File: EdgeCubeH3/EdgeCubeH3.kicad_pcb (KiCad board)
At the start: 2 copper layers, 52 x 52 mm, 19 parts, among them U1 H3, U2 K4B4G1646Q

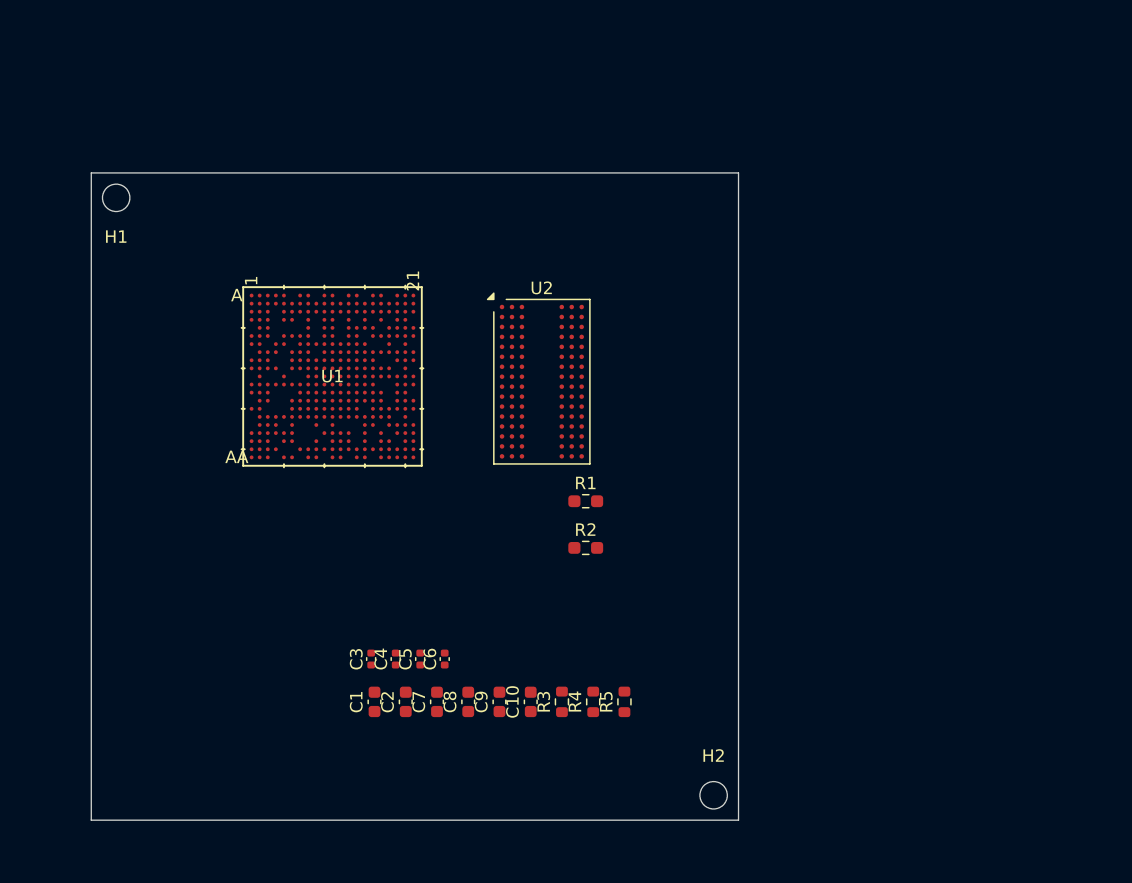
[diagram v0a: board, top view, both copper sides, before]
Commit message: Schematic update, PCB started
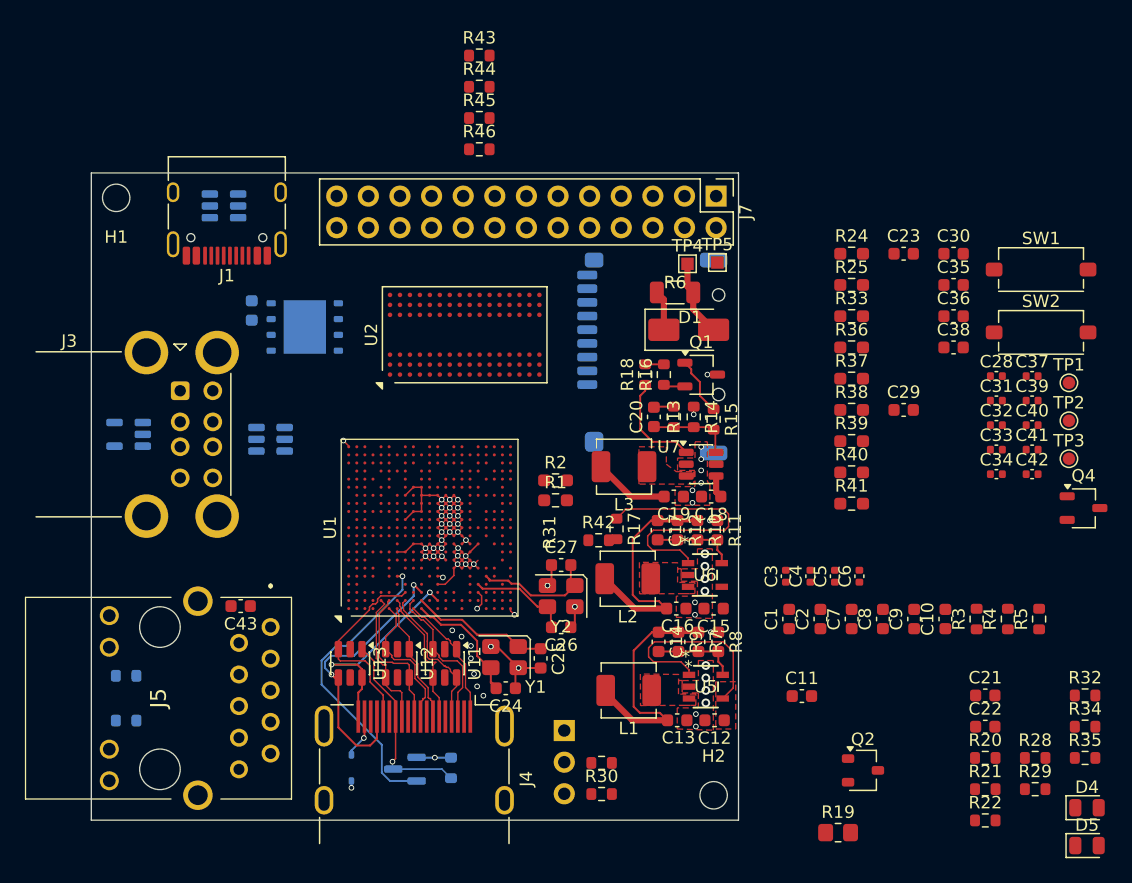
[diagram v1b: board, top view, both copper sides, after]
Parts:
- added C11: 1u, Capacitor_SMD:C_0603_1608Metric, F.Cu at (184.1, 120.0)
- added C12: 10u, Capacitor_SMD:C_0603_1608Metric, F.Cu at (177.1, 122.0)
- added C13: 10u, Capacitor_SMD:C_0603_1608Metric, F.Cu at (174.1, 122.0)
- added C14: 22p, Capacitor_SMD:C_0603_1608Metric, F.Cu at (172.6, 115.7)
- added C15: 10u, Capacitor_SMD:C_0603_1608Metric, F.Cu at (177.0, 113.0)
- added C16: 10u, Capacitor_SMD:C_0603_1608Metric, F.Cu at (174.0, 113.0)
- added C17: 22p, Capacitor_SMD:C_0603_1608Metric, F.Cu at (172.5, 106.7)
- added C18: 10u, Capacitor_SMD:C_0603_1608Metric, F.Cu at (176.8, 104.0)
- added C19: 10u, Capacitor_SMD:C_0603_1608Metric, F.Cu at (173.8, 104.0)
- added C20: 15p, Capacitor_SMD:C_0603_1608Metric, F.Cu at (172.2, 97.6)
- added C21: 2u2, Capacitor_SMD:C_0603_1608Metric, F.Cu at (198.8, 120.0)
- added C22: 2u2, Capacitor_SMD:C_0603_1608Metric, F.Cu at (198.8, 122.5)
- added C23: 4u7, Capacitor_SMD:C_0603_1608Metric, F.Cu at (192.3, 84.5)
- added C24: 15p, Capacitor_SMD:C_0603_1608Metric, F.Cu at (160.3, 119.4)
- added C25: 15p, Capacitor_SMD:C_0603_1608Metric, F.Cu at (163.1, 117.0)
- added C26: 15p, Capacitor_SMD:C_0603_1608Metric, F.Cu at (164.8, 114.5)
- added C27: 15p, Capacitor_SMD:C_0603_1608Metric, F.Cu at (164.8, 109.5)
- added C28: 100n, Capacitor_SMD:C_0402_1005Metric, F.Cu at (199.7, 94.3)
- added C29: 4u7, Capacitor_SMD:C_0603_1608Metric, F.Cu at (192.3, 97.0)
- added C30: 100n, Capacitor_SMD:C_0603_1608Metric, F.Cu at (196.3, 84.5)
- added C31: 100n, Capacitor_SMD:C_0402_1005Metric, F.Cu at (199.7, 96.3)
- added C32: 100n, Capacitor_SMD:C_0402_1005Metric, F.Cu at (199.7, 98.3)
- added C33: 100n, Capacitor_SMD:C_0402_1005Metric, F.Cu at (199.7, 100.2)
- added C34: 100n, Capacitor_SMD:C_0402_1005Metric, F.Cu at (199.7, 102.2)
- added C35: 10u, Capacitor_SMD:C_0603_1608Metric, F.Cu at (196.3, 87.0)
- added C36: 10u, Capacitor_SMD:C_0603_1608Metric, F.Cu at (196.3, 89.5)
- added C37: 100n, Capacitor_SMD:C_0402_1005Metric, F.Cu at (202.6, 94.3)
- added C38: 10u, Capacitor_SMD:C_0603_1608Metric, F.Cu at (196.3, 92.0)
- added C39: 100n, Capacitor_SMD:C_0402_1005Metric, F.Cu at (202.6, 96.3)
- added C40: 100n, Capacitor_SMD:C_0402_1005Metric, F.Cu at (202.6, 98.3)
- added C41: 100n, Capacitor_SMD:C_0402_1005Metric, F.Cu at (202.6, 100.2)
- added C42: 100n, Capacitor_SMD:C_0402_1005Metric, F.Cu at (202.6, 102.2)
- added C43: 1u, Capacitor_SMD:C_0603_1608Metric, F.Cu at (139.0, 112.8)
- added C44: 1u, Capacitor_SMD:C_0603_1608Metric, B.Cu at (139.9, 89.0)
- added D1: SS12, Diode_SMD:D_SMA, F.Cu at (175.0, 90.6)
- added D2: 1N5819WS, Diode_SMD:D_SOD-323, B.Cu at (147.9, 125.8)
- added D4: LED, LED_SMD:LED_0805_2012Metric, F.Cu at (207.0, 129.0)
- added D5: LED, LED_SMD:LED_0805_2012Metric, F.Cu at (207.0, 132.0)
- added J1: USB PWR, Connector_USB:USB_C_Receptacle_HRO_TYPE-C-31-M-12, F.Cu at (137.9, 80.6)
- added J3: USB_A_Stacked, Connector_USB:USB_A_CUI_UJ2-ADH-TH_Horizontal_Stacked, F.Cu at (134.1, 95.5)
- added J4: GPDI_A, Connector_Video:HDMI_A_Molex_208658-1001_Horizontal, F.Cu at (152.9, 125.0)
- added J5: 93626-3006, rj45:936263006, F.Cu at (141.4, 114.5)
- added J6: DBG UART, Connector_PinHeader_2.54mm:PinHeader_1x03_P2.54mm_Vertical, B.Cu at (165.0, 122.8)
- added J7: GPIO, Connector_PinHeader_2.54mm:PinHeader_2x13_P2.54mm_Vertical, F.Cu at (177.2, 79.9)
- added J8: Micro_SD_Card_Det1, icepi:microSD_TF-01A, B.Cu at (172.2, 93.1)
- added L1: 2u2, Inductor_SMD:L_APV_APH0420, F.Cu at (170.2, 119.6)
- added L2: 2u2, Inductor_SMD:L_APV_APH0420, F.Cu at (170.1, 110.6)
- added L3: 2u2, Inductor_SMD:L_APV_APH0420, F.Cu at (169.8, 101.6)
- added Q1: NPN, Package_TO_SOT_SMD:TSOT-23, F.Cu at (176.0, 94.2)
- added Q2: PMOS, Package_TO_SOT_SMD:SOT-23W, F.Cu at (189.0, 126.0)
- added Q3: AO3404, Package_TO_SOT_SMD:SOT-23, B.Cu at (152.2, 125.9)
- added Q4: NPN, Package_TO_SOT_SMD:TSOT-23, F.Cu at (206.7, 104.9)
- added R10: 200K, Capacitor_SMD:C_0603_1608Metric, F.Cu at (175.7, 106.7)
- added R11: 100K, Capacitor_SMD:C_0603_1608Metric, F.Cu at (177.3, 106.7)
- added R12: 300K, Capacitor_SMD:C_0603_1608Metric, F.Cu at (174.1, 106.7)
- added R13: 10K, Resistor_SMD:R_0603_1608Metric, F.Cu at (173.8, 97.6)
- added R14: 12K, Resistor_SMD:R_0603_1608Metric, F.Cu at (175.4, 97.6)
- added R15: 33K, Resistor_SMD:R_0603_1608Metric, F.Cu at (177.0, 97.8)
- added R16: 33K, Resistor_SMD:R_0603_1608Metric, F.Cu at (173.0, 94.2)
- added R17: 10K, Resistor_SMD:R_0603_1608Metric, F.Cu at (169.2, 106.6)
- added R18: 10K, Resistor_SMD:R_0603_1608Metric, F.Cu at (171.5, 94.2)
- added R19: 100K, Resistor_SMD:R_0805_2012Metric_Pad1.20x1.40mm_HandSolder, F.Cu at (187.0, 131.0)
- added R20: 5K6, Resistor_SMD:R_0603_1608Metric, F.Cu at (198.8, 125.0)
- added R21: 2K, Resistor_SMD:R_0603_1608Metric, F.Cu at (198.8, 127.5)
- added R22: 2K, Resistor_SMD:R_0603_1608Metric, F.Cu at (198.8, 130.0)
- added R23: 30K, Resistor_SMD:R_0603_1608Metric, B.Cu at (155.9, 125.8)
- added R24: 5K6, Resistor_SMD:R_0603_1608Metric_Pad0.98x0.95mm_HandSolder, F.Cu at (188.1, 84.5)
- added R25: 470R, Resistor_SMD:R_0603_1608Metric_Pad0.98x0.95mm_HandSolder, F.Cu at (188.1, 87.0)
- added R26: 470R, Resistor_SMD:R_0603_1608Metric, B.Cu at (129.8, 122.0)
- added R27: 470R, Resistor_SMD:R_0603_1608Metric, B.Cu at (129.8, 118.4)
- added R28: 470R, Resistor_SMD:R_0603_1608Metric, F.Cu at (202.8, 125.0)
- added R29: 470R, Resistor_SMD:R_0603_1608Metric, F.Cu at (202.8, 127.5)
- added R30: 120R, Resistor_SMD:R_0603_1608Metric, F.Cu at (168.0, 127.9)
- added R31: 120R, Resistor_SMD:R_0603_1608Metric, F.Cu at (168.0, 125.4)
- added R32: 10K, Resistor_SMD:R_0603_1608Metric, F.Cu at (206.8, 120.0)
- added R33: 33R, Resistor_SMD:R_0603_1608Metric_Pad0.98x0.95mm_HandSolder, F.Cu at (188.1, 89.5)
- added R34: 47K, Resistor_SMD:R_0603_1608Metric, F.Cu at (206.8, 122.5)
- added R35: 47K, Resistor_SMD:R_0603_1608Metric, F.Cu at (206.8, 125.0)
- added R36: 56K, Resistor_SMD:R_0603_1608Metric_Pad0.98x0.95mm_HandSolder, F.Cu at (188.1, 92.0)
- added R37: 10K, Resistor_SMD:R_0603_1608Metric_Pad0.98x0.95mm_HandSolder, F.Cu at (188.1, 94.5)
- added R38: 10K, Resistor_SMD:R_0603_1608Metric_Pad0.98x0.95mm_HandSolder, F.Cu at (188.1, 97.0)
- added R39: 10K, Resistor_SMD:R_0603_1608Metric_Pad0.98x0.95mm_HandSolder, F.Cu at (188.1, 99.5)
- added R40: 51K, Resistor_SMD:R_0603_1608Metric_Pad0.98x0.95mm_HandSolder, F.Cu at (188.1, 102.1)
- added R41: 51K, Resistor_SMD:R_0603_1608Metric_Pad0.98x0.95mm_HandSolder, F.Cu at (188.1, 104.6)
- added R42: 10M, Resistor_SMD:R_0603_1608Metric, F.Cu at (167.8, 107.5)
- added R43: 3K, Resistor_SMD:R_0603_1608Metric, F.Cu at (158.2, 68.6)
- added R44: 3K, Resistor_SMD:R_0603_1608Metric, F.Cu at (158.2, 71.1)
- added R45: 3K, Resistor_SMD:R_0603_1608Metric, F.Cu at (158.2, 73.6)
- added R46: 3K, Resistor_SMD:R_0603_1608Metric, F.Cu at (158.2, 76.1)
- added R6: 10R, Resistor_SMD:R_1206_3216Metric, F.Cu at (173.9, 87.6)
- added R7: 680K, Capacitor_SMD:C_0603_1608Metric, F.Cu at (175.8, 115.7)
- added R8: 75K, Capacitor_SMD:C_0603_1608Metric, F.Cu at (177.4, 115.7)
- added R9: 680K, Capacitor_SMD:C_0603_1608Metric, F.Cu at (174.2, 115.7)
- added SW1: RST, Button_Switch_SMD:Button_6x3mm, F.Cu at (203.3, 85.8)
- added SW2: PWR, Button_Switch_SMD:Button_6x3mm, F.Cu at (203.3, 90.8)
- added TP1: UBOOT, TestPoint:TestPoint_Pad_D1.0mm, F.Cu at (205.5, 94.9)
- added TP2: PWR_KEY, TestPoint:TestPoint_Pad_D1.0mm, F.Cu at (205.5, 97.9)
- added TP3: TV, TestPoint:TestPoint_Pad_D1.0mm, F.Cu at (205.5, 101.0)
- added TP4: supercap, TestPoint:TestPoint_Pad_1.0x1.0mm, F.Cu at (174.9, 85.3)
- added TP5: gnd, TestPoint:TestPoint_Pad_1.0x1.0mm, F.Cu at (177.3, 85.2)
- added U10: USBLC6-4SC6, Package_TO_SOT_SMD:SOT-23-6, B.Cu at (141.4, 99.4)
- added U11: USBLC6-4SC6, Package_TO_SOT_SMD:SOT-23-6, F.Cu at (155.4, 117.4)
- added U12: USBLC6-4SC6, Package_TO_SOT_SMD:SOT-23-6, F.Cu at (151.6, 117.4)
- added U13: USBLC6-4SC6, Package_TO_SOT_SMD:SOT-23-6, F.Cu at (147.8, 117.4)
- added U3: USBLC6-2SC6, Package_TO_SOT_SMD:SOT-23-6, B.Cu at (137.7, 80.7)
- added U4: SY6280AAC, Package_TO_SOT_SMD:SOT-23-5, B.Cu at (130.0, 99.0)
- added U5: SY8089AAAC, SY8089:SY8089AAAC_SGY, F.Cu at (176.4, 119.3)
- added U6: SY8089AAAC, SY8089:SY8089AAAC_SGY, F.Cu at (176.3, 110.3)
- added U7: SY8032, Package_TO_SOT_SMD:SOT-23-6, F.Cu at (176.0, 101.4)
- added U8: W25Q128JVP, Package_SON:WSON-8-1EP_6x5mm_P1.27mm_EP3.4x4.3mm, B.Cu at (144.2, 90.4)
- added Y1: 24M, Crystal:Crystal_SMD_3225-4Pin_3.2x2.5mm, F.Cu at (160.2, 116.9)
- added Y2: 32K, Crystal:Crystal_SMD_3225-4Pin_3.2x2.5mm, F.Cu at (164.8, 112.0)
- U1: footprint Lib:BGA347_H3_AWT-M -> cm0:FBGA-347_14x14mm_Layout21x21_P0.65mm
- moved C2 34.0 mm to (185.6, 113.8)
- moved C9 34.0 mm to (193.1, 113.8)
- moved C1 34.0 mm to (183.1, 113.8)
- moved C10 34.0 mm to (195.6, 113.8)
- moved C3 34.0 mm to (182.8, 110.4)
- moved C4 34.0 mm to (184.8, 110.4)
- moved C5 34.0 mm to (186.7, 110.4)
- moved C6 34.0 mm to (188.7, 110.4)
- moved C7 34.0 mm to (188.1, 113.8)
- moved C8 34.0 mm to (190.6, 113.8)
- moved R3 34.0 mm to (198.1, 113.8)
- moved R4 34.0 mm to (200.6, 113.8)
- moved R5 34.0 mm to (203.2, 113.8)
- moved U1 14.4 mm to (154.2, 106.5), turned to 90 degrees
- moved U2 7.26 mm to (157.0, 91.0), turned to 90 degrees
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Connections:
- net VDD_DRAM renamed +1V35
- U1 pad A19: unconnected-(U1F-PF1-PadA19) -> /SoC/SDC0_D0
- U1 pad A2: unconnected-(U1D-EPHY_LINK_LED-PadA2) -> /SoC/EPHY_LINK_LED
- U1 pad A21: Net-(U1B-GND-PadA21) -> GND
- U1 pad A3: unconnected-(U1D-EPHY_TXN-PadA3) -> /SoC/EPHY_TX-
- U1 pad A4: unconnected-(U1D-EPHY_RXN-PadA4) -> /SoC/EPHY_RX-
- U1 pad A5: unconnected-(U1E-USB_D0+-PadA5) -> USB_D0+
- U1 pad A7: unconnected-(U1E-USB_D2+-PadA7) -> USB_D2+
- U1 pad A8: unconnected-(U1E-USB_D2--PadA8) -> USB_D2-
- U1 pad AA1: Net-(U1B-GND-PadA21) -> GND
- U1 pad AA6: unconnected-(U1G-NMI-PadAA6) -> Net-(U1G-NMI)
- U1 pad B13: unconnected-(U1F-PA18-PadB13) -> TWI1_SCK
- U1 pad B14: unconnected-(U1F-PA19-PadB14) -> TWI1_SDA
- U1 pad B15: unconnected-(U1C-PC3-PadB15) -> SPI0_CS
- U1 pad B16: unconnected-(U1C-PC2-PadB16) -> SPI0_CLK
- U1 pad B3: unconnected-(U1D-EPHY_TXP-PadB3) -> /SoC/EPHY_TX+
- U1 pad B4: unconnected-(U1D-EPHY_RXP-PadB4) -> /SoC/EPHY_RX+
- U1 pad B5: unconnected-(U1E-USB_D0--PadB5) -> USB_D0-
- U1 pad B6: unconnected-(U1E-USB_D1+-PadB6) -> USB_D1+
- U1 pad B7: unconnected-(U1E-USB_D1--PadB7) -> USB_D1-
- U1 pad C13: unconnected-(U1F-PA12-PadC13) -> TWI0_SDA
- U1 pad C14: unconnected-(U1F-PA17-PadC14) -> STATUS_LED
- U1 pad C15: unconnected-(U1C-PC0-PadC15) -> SPI0_MOSI
- U1 pad C16: unconnected-(U1C-PC1-PadC16) -> SPI0_MISO
- U1 pad C20: unconnected-(U1F-PF5-PadC20) -> /SoC/SDC0_D2
- U1 pad D11: unconnected-(U1F-PA0-PadD11) -> UART2_TX
- U1 pad D15: unconnected-(U1F-PA16-PadD15) -> SPI1_MISO
- U1 pad D19: unconnected-(U1F-PF0-PadD19) -> /SoC/SDC0_D1
- U1 pad D20: unconnected-(U1F-PF2-PadD20) -> Net-(U1F-PF2)
- U1 pad D3: unconnected-(U1C-PG7-PadD3) -> UART1_RX
- U1 pad D5: unconnected-(U1F-PA1-PadD5) -> UART2_RX
- U1 pad D6: unconnected-(U1F-PA2-PadD6) -> UART2_RTS
- U1 pad D8: unconnected-(U1F-PA7-PadD8) -> PA7
- U1 pad E11: unconnected-(U1F-PA10-PadE11) -> PA10
- U1 pad E13: unconnected-(U1F-PA3-PadE13) -> UART2_CTS
- U1 pad E14: unconnected-(U1F-PA6-PadE14) -> PA6
- U1 pad E15: unconnected-(U1F-PA13-PadE15) -> SPI1_CS
- U1 pad E2: unconnected-(U1D-GPDI_CLK--PadE2) -> /SoC/GPDI_CLK-
- U1 pad E21: unconnected-(U1F-PF4-PadE21) -> /SoC/SDC0_D3
- U1 pad F1: unconnected-(U1D-GPDI_D0--PadF1) -> /SoC/GPDI_D0-
- U1 pad F10: unconnected-(U1D-TVOUT-PadF10) -> Net-(U1D-TVOUT)
- U1 pad F11: unconnected-(U1F-PA11-PadF11) -> TWI0_SCK
- U1 pad F14: unconnected-(U1F-PA15-PadF14) -> SPI1_MOSI
- U1 pad F18: unconnected-(U1F-PF3-PadF18) -> /SoC/SDC0_CMD
- U1 pad F2: unconnected-(U1D-GPDI_CLK+-PadF2) -> /SoC/GPDI_CLK+
- U1 pad F5: unconnected-(U1F-PA4-PadF5) -> UART0_TX
- U1 pad F6: unconnected-(U1D-EPHY_RTX-PadF6) -> Net-(U1D-EPHY_RTX)
- U1 pad F7: unconnected-(U1D-EPHY_SPD_LED-PadF7) -> /SoC/EPHY_SPD_LED
- U1 pad F8: unconnected-(U1D-EPHY_VDD-PadF8) -> +1V2
- U1 pad G1: unconnected-(U1D-GPDI_D0+-PadG1) -> /SoC/GPDI_D0+
- U1 pad G10: unconnected-(U1B-VDD-EFUSE-PadG10) -> Net-(U1B-VDD-EFUSE)
- U1 pad G11: unconnected-(U1E-VCC_USB-PadG11) -> VCC_IO
- U1 pad G12: unconnected-(U1F-PA14-PadG12) -> SPI1_CLK
- U1 pad G13: unconnected-(U1B-VCC-IO-PadG13) -> VCC_IO
- U1 pad G14: unconnected-(U1B-VCC-IO-PadG14) -> VCC_IO
- U1 pad G15: unconnected-(U1B-VCC-IO-PadG15) -> VCC_IO
- U1 pad G18: unconnected-(U1F-PF6-PadG18) -> /SoC/SDC0_DET
- U1 pad G2: unconnected-(U1D-GPDI_D1--PadG2) -> /SoC/GPDI_D1-
- U1 pad G4: unconnected-(U1C-PG6-PadG4) -> UART1_TX
- U1 pad G5: unconnected-(U1D-GPDI_CEC-PadG5) -> /SoC/GPDI_CEC
- U1 pad G7: unconnected-(U1D-EPHY_VCC-PadG7) -> +3V3
- U1 pad G8: Net-(U1B-GND-PadA21) -> GND
- U1 pad G9: unconnected-(U1D-V33_TV-PadG9) -> +3V3
- U1 pad H10: unconnected-(U1B-VDD-SYS-PadH10) -> +1V2
- U1 pad H11: unconnected-(U1B-VDD-EFUSEEBP-PadH11) -> +3V3
- U1 pad H12: Net-(U1B-GND-PadA21) -> GND
- U1 pad H13: unconnected-(U1B-VCC-IO-PadH13) -> VCC_IO
- U1 pad H14: unconnected-(U1B-VCC-IO-PadH14) -> VCC_IO
- U1 pad H15: Net-(U1B-GND-PadA21) -> GND
- U1 pad H2: unconnected-(U1D-GPDI_D1+-PadH2) -> /SoC/GPDI_D1+
- U1 pad H3: unconnected-(U1D-GPDI_SCL-PadH3) -> /SoC/GPDI_SCL
- U1 pad H6: unconnected-(U1F-PA5-PadH6) -> UART0_RX
- U1 pad H7: unconnected-(U1C-VCC-PG-PadH7) -> VCC_IO
- U1 pad H8: unconnected-(U1D-GND_TV-PadH8) -> GND
- U1 pad J1: unconnected-(U1D-GPDI_D2+-PadJ1) -> /SoC/GPDI_D2+
- U1 pad J10: unconnected-(U1B-VDD-SYS-PadJ10) -> +1V2
- U1 pad J11: unconnected-(U1B-VDD-SYS-PadJ11) -> +1V2
- U1 pad J12: unconnected-(U1B-VDD-SYS-PadJ12) -> +1V2
- U1 pad J13: Net-(U1B-GND-PadA21) -> GND
- U1 pad J14: unconnected-(U1B-VCC-IO-PadJ14) -> VCC_IO
- U1 pad J15: unconnected-(U1F-VCC_PD-PadJ15) -> VCC_IO
- U1 pad J16: Net-(U1B-GND-PadA21) -> GND
- U1 pad J2: unconnected-(U1D-GPDI_D2--PadJ2) -> /SoC/GPDI_D2-
- U1 pad J6: unconnected-(U1D-GPDI_VCC-PadJ6) -> +3V3
- U1 pad J7: unconnected-(U1B-VDD-CPUS-PadJ7) -> +1V2
- U1 pad J8: unconnected-(U1B-VDD-CPUS-PadJ8) -> +1V2
- U1 pad J9: Net-(U1B-GND-PadA21) -> GND
- U1 pad K1: unconnected-(U1G-X24MOUT-PadK1) -> Net-(U1G-X24MOUT)
- U1 pad K10: unconnected-(U1B-VDD-SYS-PadK10) -> +1V2
- U1 pad K11: unconnected-(U1B-VDD-SYS-PadK11) -> +1V2
- U1 pad K12: unconnected-(U1B-VDD-SYS-PadK12) -> +1V2
- U1 pad K13: Net-(U1B-GND-PadA21) -> GND
- U1 pad K14: Net-(U1B-GND-PadA21) -> GND
- U1 pad K15: Net-(U1B-GND-PadA21) -> GND
- U1 pad K16: Net-(U1B-GND-PadA21) -> GND
- U1 pad K2: unconnected-(U1G-X24MIN-PadK2) -> Net-(U1G-X24MIN)
- U1 pad K3: unconnected-(U1D-GPDI_SDA-PadK3) -> /SoC/GPDI_SDA
- U1 pad K6: unconnected-(U1G-VCC_RTC-PadK6) -> +3V3
- U1 pad K7: Net-(U1B-GND-PadA21) -> GND
- U1 pad K8: Net-(U1B-GND-PadA21) -> GND
- U1 pad K9: Net-(U1B-GND-PadA21) -> GND
- U1 pad L10: unconnected-(U1B-VDD-SYS-PadL10) -> +1V2
- U1 pad L11: unconnected-(U1B-VDD-SYS-PadL11) -> +1V2
- U1 pad L12: unconnected-(U1B-VDD-SYS-PadL12) -> +1V2
- U1 pad L13: unconnected-(U1B-VDD-SYS-PadL13) -> +1V2
- U1 pad L14: unconnected-(U1B-VDD-SYS-PadL14) -> +1V2
- U1 pad L15: Net-(U1B-GND-PadA21) -> GND
- U1 pad L8: Net-(U1B-GND-PadA21) -> GND
- U1 pad L9: Net-(U1B-GND-PadA21) -> GND
- U1 pad M10: Net-(U1B-GND-PadA21) -> GND
- U1 pad M11: Net-(U1B-GND-PadA21) -> GND
- U1 pad M12: Net-(U1B-GND-PadA21) -> GND
- U1 pad M13: Net-(U1B-GND-PadA21) -> GND
- U1 pad M14: Net-(U1B-GND-PadA21) -> GND
- U1 pad M15: Net-(U1B-GND-PadA21) -> GND
- U1 pad M2: unconnected-(U1D-GPDI_HPD-PadM2) -> /SoC/GPDI_HPD
- U1 pad M4: unconnected-(U1G-RTC_VIO-PadM4) -> +1V2
- U1 pad M5: unconnected-(U1D-GPDI_GND-PadM5) -> GND
- U1 pad M6: unconnected-(U1F-PL9-PadM6) -> PWR_DRAM_EN
- U1 pad M7: Net-(U1B-GND-PadA21) -> GND
- U1 pad M8: Net-(U1B-GND-PadA21) -> GND
- U1 pad M9: Net-(U1B-GND-PadA21) -> GND
- U1 pad N10: Net-(U1B-GND-PadA21) -> GND
- U1 pad N11: Net-(U1B-GND-PadA21) -> GND
- U1 pad N12: Net-(U1B-GND-PadA21) -> GND
- U1 pad N13: Net-(U1B-GND-PadA21) -> GND
- U1 pad N14: Net-(U1B-GND-PadA21) -> GND
- U1 pad N15: Net-(U1B-GND-PadA21) -> GND
- U1 pad N2: unconnected-(U1F-PL4-PadN2) -> Net-(U1F-PL4)
- U1 pad N3: unconnected-(U1G-VCC_PLL-PadN3) -> +3V3
- U1 pad N7: Net-(U1B-GND-PadA21) -> GND
- U1 pad N8: unconnected-(U1B-VDD-CPUX-PadN8) -> +1V2
- U1 pad N9: Net-(U1B-GND-PadA21) -> GND
- U1 pad P10: Net-(U1B-GND-PadA21) -> GND
- U1 pad P11: Net-(U1B-GND-PadA21) -> GND
- U1 pad P12: Net-(U1B-GND-PadA21) -> GND
- U1 pad P13: Net-(U1B-GND-PadA21) -> GND
- U1 pad P14: Net-(U1B-GND-PadA21) -> GND
- U1 pad P15: Net-(U1B-GND-PadA21) -> GND
- U1 pad P6: unconnected-(U1B-VDD-CPUX-PadP6) -> +1V2
- U1 pad P7: unconnected-(U1B-VDD-CPUX-PadP7) -> +1V2
- U1 pad P8: unconnected-(U1B-VDD-CPUX-PadP8) -> +1V2
- U1 pad P9: unconnected-(U1B-VDD-CPUX-PadP9) -> +1V2
- U1 pad R1: unconnected-(U1F-PL3-PadR1) -> Net-(U1F-PL3)
- U1 pad R10: Net-(U1B-GND-PadA21) -> GND
- U1 pad R11: Net-(U1B-GND-PadA21) -> GND
- U1 pad R12: Net-(U1B-GND-PadA21) -> GND
- U1 pad R13: Net-(U1B-GND-PadA21) -> GND
- U1 pad R14: Net-(U1B-GND-PadA21) -> GND
- U1 pad R2: unconnected-(U1F-PL5-PadR2) -> VCC_IO_EN
- U1 pad R6: unconnected-(U1B-VDD-CPUX-PadR6) -> +1V2
- U1 pad R7: unconnected-(U1B-VDD-CPUX-PadR7) -> +1V2
- U1 pad R8: unconnected-(U1B-VDD-CPUX-PadR8) -> +1V2
- U1 pad R9: Net-(U1B-GND-PadA21) -> GND
- U1 pad T10: unconnected-(U1G-VDD-CPUFB-PadT10) -> PWR_CPUFB
- U1 pad T11: Net-(U1B-GND-PadA21) -> GND
- U1 pad T2: unconnected-(U1F-PL8-PadT2) -> PWR_STB_EN
- U1 pad T4: unconnected-(U1F-PL6-PadT4) -> CPUX_VSET
- U1 pad T6: unconnected-(U1B-VDD-CPUX-PadT6) -> +1V2
- U1 pad T7: unconnected-(U1B-VDD-CPUX-PadT7) -> +1V2
- U1 pad T8: unconnected-(U1B-VDD-CPUX-PadT8) -> +1V2
- U1 pad T9: unconnected-(U1G-GND-CPUFB-PadT9) -> GND
- U1 pad U3: unconnected-(U1H-AGND-PadU3) -> GND
- U1 pad U4: unconnected-(U1G-X32KOUT-PadU4) -> Net-(U1G-X32KOUT)
- U1 pad U6: unconnected-(U1B-VDD-CPUX-PadU6) -> +1V2
- U1 pad U9: unconnected-(U1B-VDD-CPUX-PadU9) -> +1V2
- U1 pad V2: unconnected-(U1F-PL10-PadV2) -> PWR_LED
- U1 pad V3: unconnected-(U1H-AVCC-PadV3) -> +3V3
- U1 pad V5: unconnected-(U1G-X32KIN-PadV5) -> Net-(U1G-X32KIN)
- U1 pad V6: unconnected-(U1G-RESET-PadV6) -> /SoC/RESET
- U1 pad W6: unconnected-(U1G-UBOOT-PadW6) -> Net-(U1G-UBOOT)
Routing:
- net GND: track 0.00 -> 64.4 mm, vias 0 -> 53
- net /SoC/GPDI_CEC: track 0.00 -> 24.5 mm, vias 0 -> 1
- net /SoC/GPDI_SDA: track 0.00 -> 22.7 mm, vias 0 -> 2
- net PWR_DRAM_EN: track 0.00 -> 22.1 mm
- net VBUS: track 0.00 -> 21.8 mm, vias 0 -> 1
- net +3V3: track 0.00 -> 21.5 mm
- net +1V35: track 0.00 -> 20.1 mm
- net +1V2: track 0.00 -> 19.8 mm, vias 0 -> 6
- net /SoC/GPDI_HPD: track 0.00 -> 17.7 mm, vias 0 -> 2
- net /SoC/GPDI_SCL: track 0.00 -> 16.0 mm
- net /ports/CEC: track 0.00 -> 15.8 mm, vias 0 -> 1
- net /SoC/GPDI_D2-: track 0.00 -> 12.2 mm
- net /SoC/GPDI_D1+: track 0.00 -> 11.9 mm
- net /SoC/GPDI_CLK+: track 0.00 -> 11.9 mm
- net /SoC/GPDI_D0-: track 0.00 -> 11.5 mm
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- added copper zone on F.Cu, net GND
- added copper zone on In1.Cu, net GND
- added copper zone on In4.Cu, net GND
- added copper zone on F.Cu, net Net-(U5-LX)
- added copper zone on F.Cu, net Net-(U6-LX)
- added copper zone on F.Cu, net Net-(U7-LX)
- added copper zone on F.Cu, net VBUS
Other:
- copper layers 2 -> 6

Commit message: PCB design at ~90%
- re-arrangement of components
- connecting dram
- connecting ports
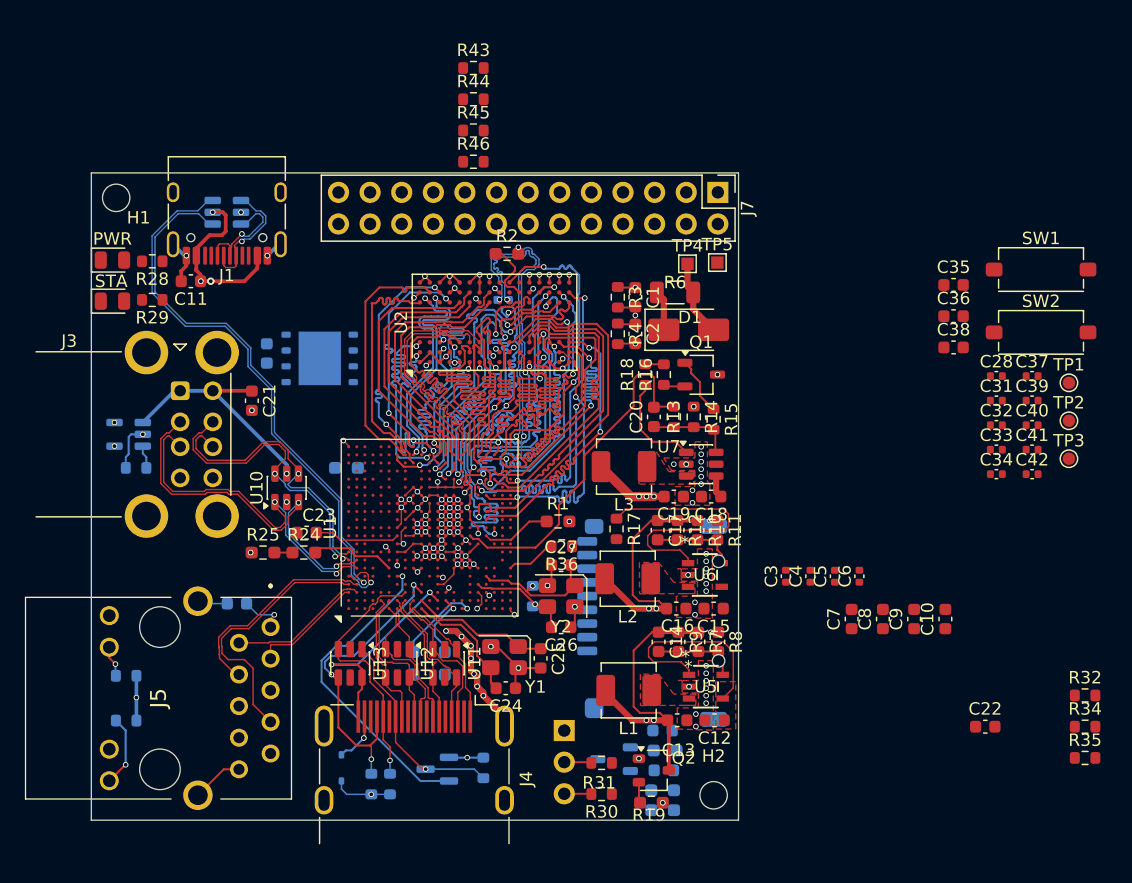
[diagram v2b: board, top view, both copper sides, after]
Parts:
- C29, C30, C43, Q4, R20, R21, R22, R33, R37, R38, R39, R40, R41, R42: moved to B.Cu
- D4: value LED -> PWR
- D5: value LED -> STA
- R19: footprint Resistor_SMD:R_0805_2012Metric_Pad1.20x1.40mm_HandSolder -> Resistor_SMD:R_0603_1608Metric_Pad0.98x0.95mm_HandSolder
- R36: footprint Resistor_SMD:R_0603_1608Metric_Pad0.98x0.95mm_HandSolder -> Resistor_SMD:R_0603_1608Metric
- R5: footprint Resistor_SMD:R_0603_1608Metric -> Resistor_SMD:R_0402_1005Metric; moved to B.Cu
- U10: moved to F.Cu
- moved D4 89.8 mm to (128.7, 85.0)
- moved D5 89.7 mm to (128.7, 88.3)
- moved R28 81.4 mm to (131.9, 85.1), turned to 180 degrees
- moved R29 81.1 mm to (131.9, 88.2), turned to 180 degrees
- moved R20 72.1 mm to (130.6, 101.7)
- moved C21 63.5 mm to (139.9, 96.3), turned to -90 degrees
- moved C11 59.3 mm to (135.0, 86.7), turned to 180 degrees
- moved C23 52.9 mm to (144.3, 106.9), turned to 180 degrees
- moved R25 51.9 mm to (140.8, 108.5)
- moved R24 50.1 mm to (144.1, 108.5)
- moved R5 50.1 mm to (160.1, 88.2), turned to 0 degrees
- moved R21 49.3 mm to (149.5, 127.1), turned to -90 degrees
- moved R22 47.9 mm to (151.0, 127.1), turned to 90 degrees
- moved C30 44.9 mm to (172.9, 122.8)
- moved Q4 42.8 mm to (169.0, 125.1), turned to 180 degrees
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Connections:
- net Net-(J1-D+-PadA6) renamed /power/USB+
- net Net-(J1-D--PadA7) renamed /power/USB-
- U2 pad A3: /SoC/SDQ15 -> /SoC/SDQ12
- U2 pad A7: /SoC/SDQ12 -> /SoC/SDQ8
- U2 pad B8: /SoC/SDQ14 -> /SoC/SDQ9
- U2 pad C2: /SoC/SDQ11 -> /SoC/SDQ15
- U2 pad C3: /SoC/SDQ9 -> /SoC/SDQ14
- U2 pad D7: /SoC/SDQ8 -> /SoC/SDQ11
- U2 pad E3: /SoC/SDQ0 -> /SoC/SDQ5
- U2 pad F2: /SoC/SDQ2 -> /SoC/SDQ6
- U2 pad F7: /SoC/SDQ1 -> /SoC/SDQ2
- U2 pad F8: /SoC/SDQ3 -> /SoC/SDQ0
- U2 pad G2: /SoC/SDQ6 -> /SoC/SDQ3
- U2 pad H3: /SoC/SDQ4 -> /SoC/SDQ7
- U2 pad H7: /SoC/SDQ7 -> /SoC/SDQ4
- U2 pad H8: /SoC/SDQ5 -> /SoC/SDQ1
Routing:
- net USB_D0-: track 0.00 -> 45.9 mm, vias 0 -> 1
- net USB_D0+: track 0.00 -> 43.8 mm, vias 0 -> 1
- net GND: track 64.4 -> 106.2 mm, vias 53 -> 98
- net VREF: track 0.00 -> 36.3 mm, vias 0 -> 4
- net USB_D1-: track 0.00 -> 29.7 mm, vias 0 -> 2
- net USB_D1+: track 0.00 -> 29.2 mm, vias 0 -> 2
- net /SoC/SWE: track 0.00 -> 27.3 mm
- net /SoC/SBA0: track 0.00 -> 26.9 mm
- net /SoC/SBA2: track 0.00 -> 26.9 mm
- net /SoC/SCK+: track 0.00 -> 26.9 mm, vias 0 -> 2
- net /SoC/SCK-: track 0.00 -> 26.9 mm, vias 0 -> 2
- net /SoC/SA5: track 0.00 -> 26.9 mm
- net /SoC/SA3: track 0.00 -> 26.8 mm
- net PWR_CPUFB: track 1.62 -> 28.3 mm
- net /SoC/SA15: track 0.00 -> 26.0 mm, vias 0 -> 2
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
